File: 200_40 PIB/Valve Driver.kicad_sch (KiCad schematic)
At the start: 46 parts, among them J4 53398-0671, Q10 IRF7832, U1 LT3065EDDPBF, U18 74LVC2G14, U2 MIC4424YM, U3 MIC4424YM, U6 LM1117MP-3.3, U9 74LVC2G17

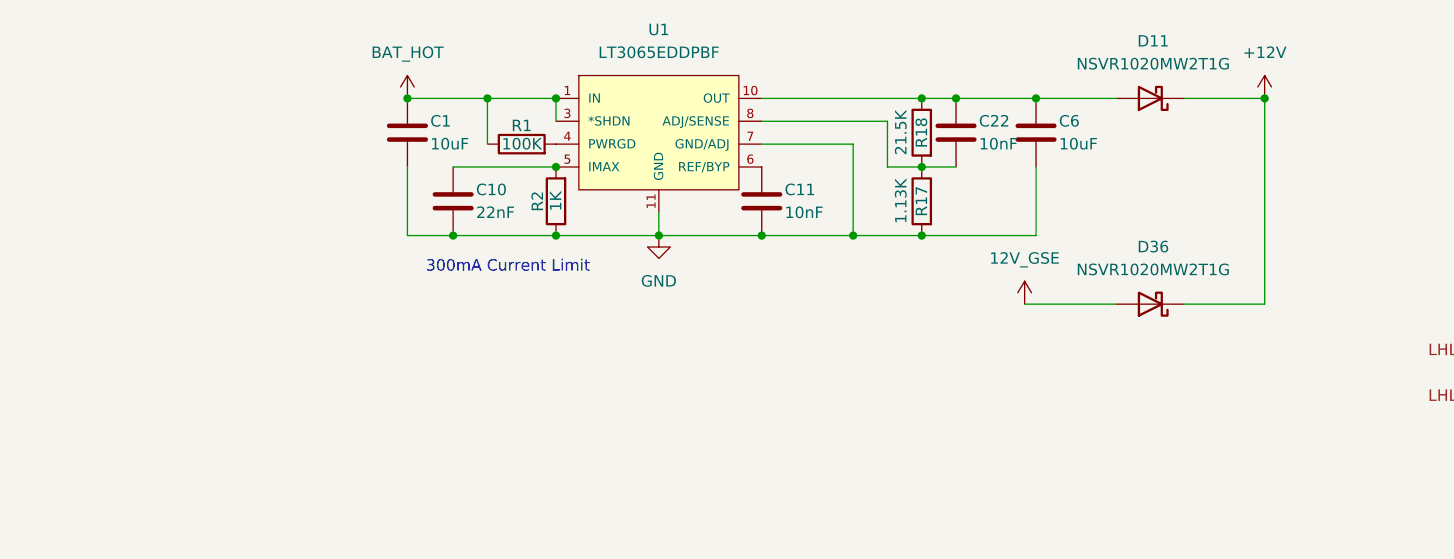
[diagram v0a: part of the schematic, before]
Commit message: clod
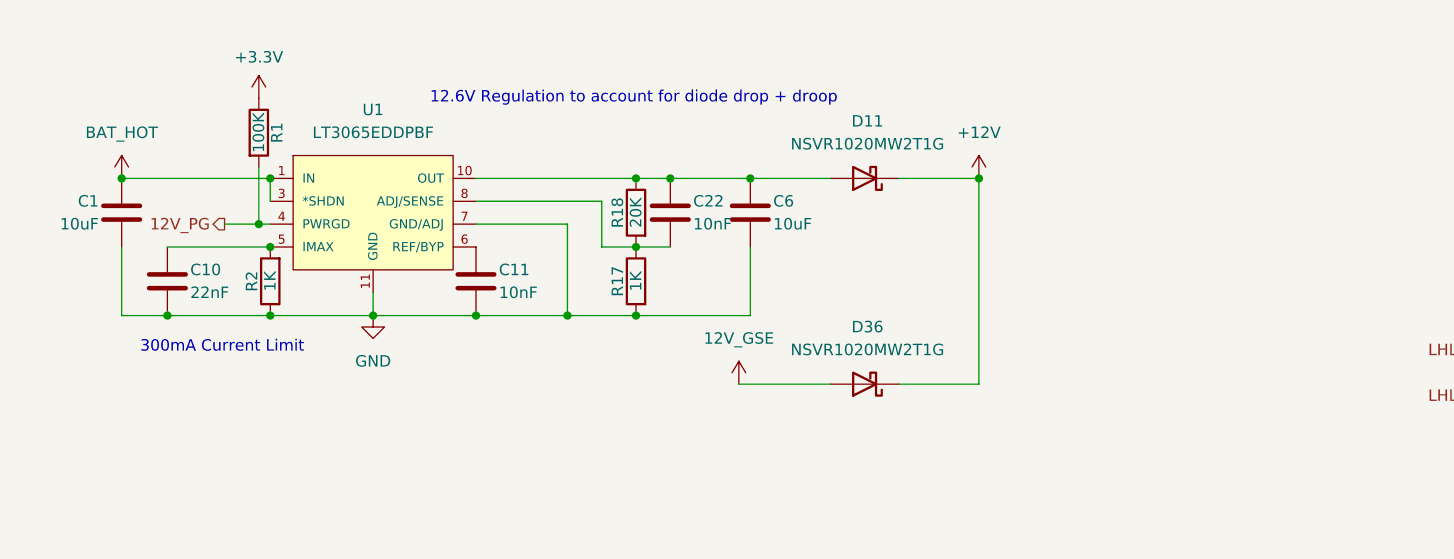
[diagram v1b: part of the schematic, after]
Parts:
- R17: value 1.13K -> 1K
- R18: value 21.5K -> 20K
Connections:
- net BAT_HOT: no longer R1.1
- net 12V_PG: now reaches R1.2, U1.4 (PWRGD)
- new net +3.3V: R1.1
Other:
- note added: "12.6V Regulation to account for diode drop + droop"
- moved on the sheet: C1, C10, C11, C22, C6, D11, D36, R1, R17, R18, R2, U1
